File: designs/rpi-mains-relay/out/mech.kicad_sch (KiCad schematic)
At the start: 12 parts

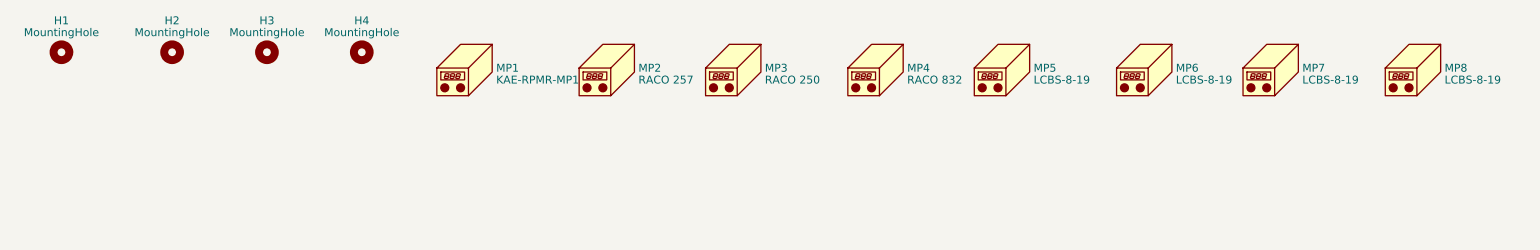
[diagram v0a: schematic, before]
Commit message: designs: work-in-progress (Prius encoding and relay-board rework under way)
Co-Authored-By: Claude Opus 5.5 <noreply@anthropic.com>
Claude-Session: https://claude.ai/code/session_01VFJn9VbX8h27kf4LpLwEtn
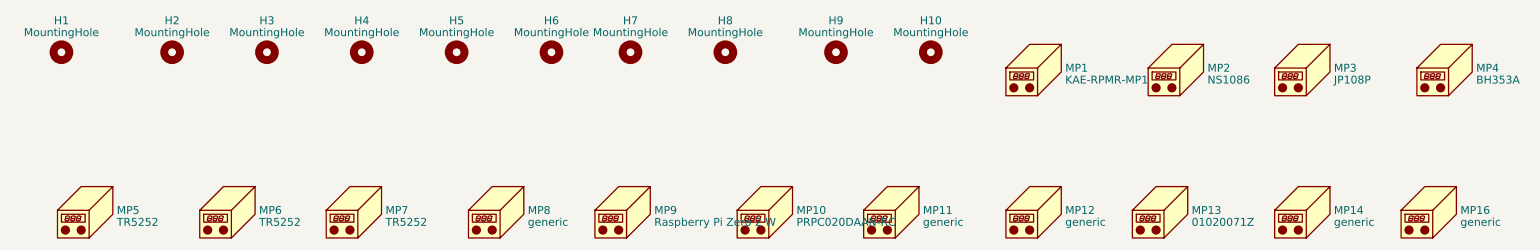
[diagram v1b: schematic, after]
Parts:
- added H10, H7, H8, H9: MountingHole, MountingHole:MountingHole_2.7mm_M2.5, symbol Mechanical:MountingHole
- added H5, H6: MountingHole, MountingHole:MountingHole_3.2mm_M3, symbol Mechanical:MountingHole
- added MP10: PRPC020DAAN-RC, symbol Mechanical:Housing
- added MP11, MP12, MP14, MP16: generic, symbol Mechanical:Housing
- added MP13: 01020071Z, symbol Mechanical:Housing
- added MP9: Raspberry Pi Zero 2 W, symbol Mechanical:Housing
- H1, H2, H3, H4: footprint MountingHole:MountingHole_4mm -> MountingHole:MountingHole_3.2mm_M3
- MP1: Manufacturer custom (die-cut to drawing, TBD) -> custom (die-cut and folded to drawing, TBD)
- MP2: value RACO 257 -> NS1086; MPN RACO 257 -> NS1086; Manufacturer Hubbell RACO -> ABB (Carlon) Circuit Safe
- MP3: value RACO 250 -> JP108P; MPN RACO 250 -> JP108P; Manufacturer Hubbell RACO -> ABB (Carlon)
- MP4: value RACO 832 -> BH353A; MPN RACO 832 -> BH353A; Manufacturer Hubbell RACO -> ABB (Carlon) Superblue
- MP5, MP6, MP7: value LCBS-8-19 -> TR5252; MPN LCBS-8-19 -> TR5252; Manufacturer Essentra Components (Richco) -> Legrand Pass & Seymour
- MP8: value LCBS-8-19 -> generic; MPN LCBS-8-19 -> (none); Manufacturer Essentra Components (Richco) -> generic
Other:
- title: Mounting holes, SELV cover and box parts (BOM only) -> Holes; partition; enclosures, receptacles, Pi and hardware (BOM only)
- moved on the sheet: MP1, MP2, MP3, MP4, MP5, MP6, MP7, MP8
